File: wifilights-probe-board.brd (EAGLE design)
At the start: 50.8 x 25.4 mm, 18 parts, among them J1 22-05-7028-02, U1 FT232R

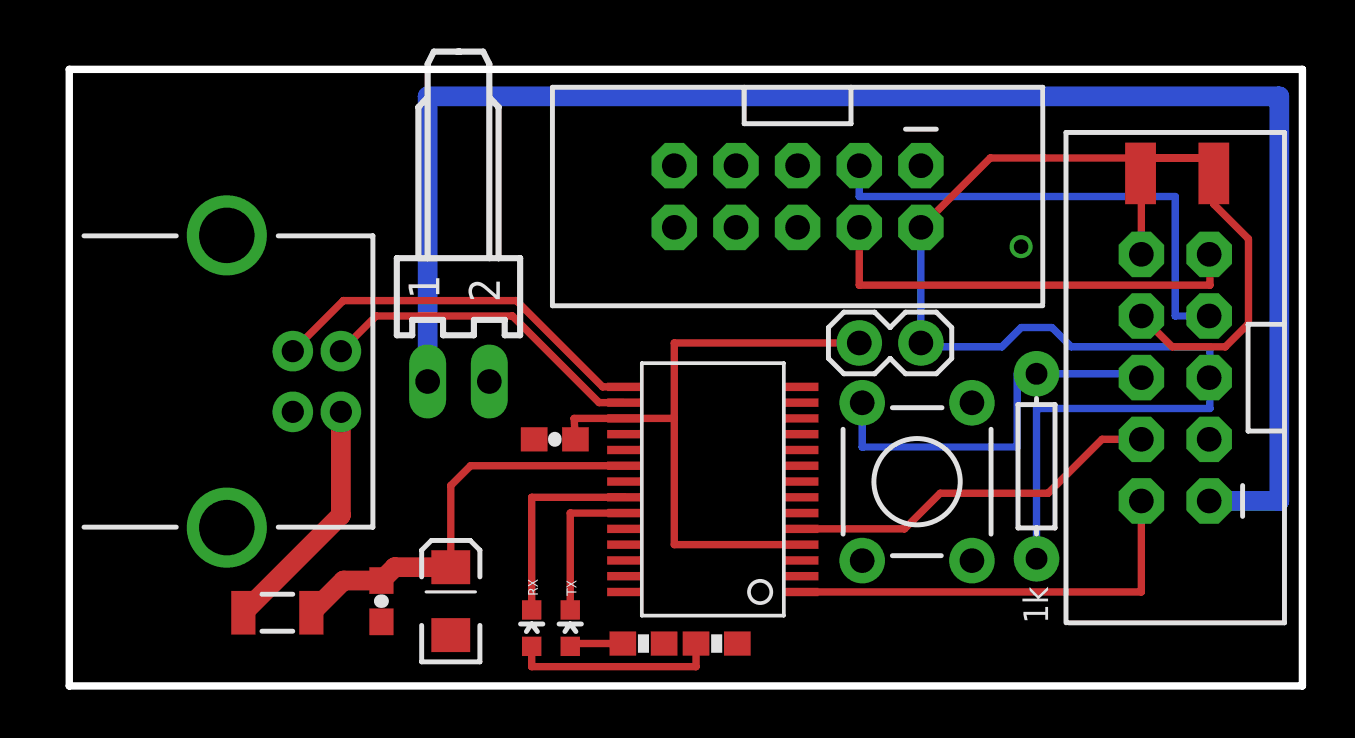
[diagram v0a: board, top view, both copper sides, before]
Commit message: Mk6 complete & DRC'd
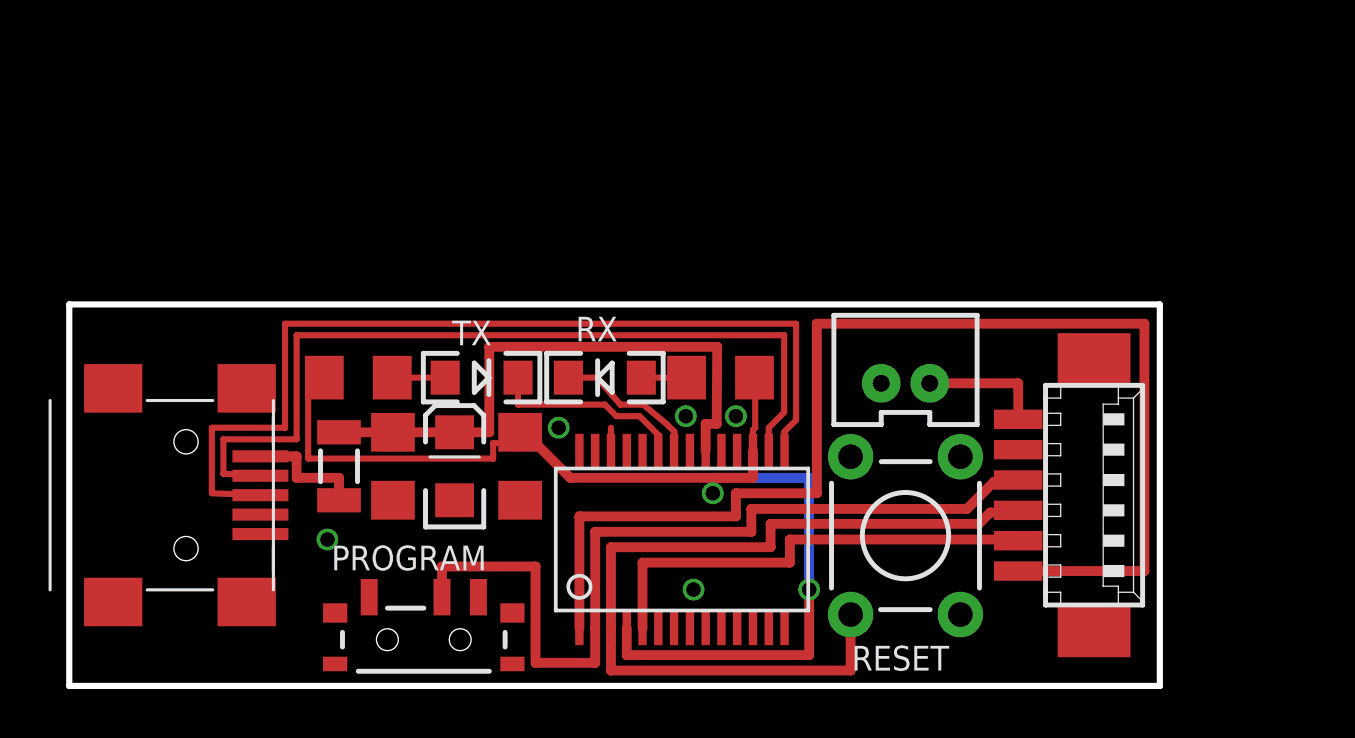
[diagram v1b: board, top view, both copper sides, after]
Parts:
- removed J1: 22-05-7028-02, con-molex:7395-02
- removed JP2: (no value), SparkFun-Connectors:2X5-SHROUDED_LOCK
- removed JP3: (no value), SparkFun-Retired:1X02
- removed JP4: USB-B, SparkFun-Connectors:USB-B-PTH
- removed R4: 1k, SparkFun-Passives:AXIAL-0.3
- removed S2: SWITCH-MOMENTARY-2PTH, SparkFun-Electromechanical:TACTILE-PTH
- removed SH1, SH2: SHORT-HT5, shorts-old:SHORT_TOP-50
- added CN1: (no value), adafruit:USB-MINIB
- added PROGRAM: (no value), SparkFun-Electromechanical:SWITCH-SPST-SMD-A
- added RESET: SWITCH-MOMENTARY-2PTH, SparkFun-Electromechanical:TACTILE-PTH
- added X1: 53261-06, con-molex:53261-06
- C1, C2: device SparkFun-Capacitors:0603-CAP -> SparkFun-Passives:1206
- JP1: value (none) -> 12V DC; device SparkFun-Connectors:2X5-SHROUDED -> SparkFun-Connectors:JST-2-PTH-VERT
- R1, R2: device SparkFun-Resistors:0603-RES -> SparkFun-Passives:1206
- RX: value Green -> GREEN; device SparkFun-LED:LED-0603 -> SparkFun-LED:LED-1206
- TX: value Red -> RED; device SparkFun-LED:LED-0603 -> SparkFun-LED:LED-1206
- moved R1 16.1 mm to (11.9, 12.7), turned to 180 degrees
- moved R2 11.0 mm to (26.8, 12.7)
- moved TX 10.9 mm to (17.0, 12.7)
- moved RX 10.8 mm to (22.1, 12.7), turned to 180 degrees
- moved JP1 8.41 mm to (34.4, 13.0), turned to 0 degrees
- moved F1 6.55 mm to (11.1, 9.05), turned to 90 degrees
- moved C2 5.58 mm to (13.3, 9.05)
- moved C5 5.56 mm to (15.9, 9.05)
- moved U1 2.42 mm to (25.2, 6.03), turned to 0 degrees
- moved C1 1.81 mm to (18.6, 9.05), turned to 270 degrees
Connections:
- removed net 3.3V-INT: C1.1, JP3.2, U1.17, U1.4
- removed net 5V: JP1.1
- removed net CH_PD: JP2.10, SH2.1
- removed net GPIO0: JP2.6, R4.P$1, S2.3
- removed net GPIO2: JP2.8, SH1.1
- removed net N$4: R1.2
- removed net N$5: R2.2
- removed net P_RED: JP1.8
- removed net P_WHITE: JP1.6
- removed net RED: JP1.7
- removed net SCL: JP1.3, JP2.7
- removed net SDA: JP1.4, JP2.9
- removed net WHITE: JP1.5
- net 12V: now also JP1.2, X1.6; no longer J1.1, JP2.1
- net 3.3V: now also C1.1, R1.2, R2.2, U1.17, U1.4; no longer JP1.2, JP2.5, JP3.1, R4.P$2, SH1.2, SH2.2
- net DTR: now also PROGRAM.2, X1.4
- net GND: now also CN1.GND, JP1.1, PROGRAM.3, RESET.3, X1.5; no longer J1.2, JP1.10, JP1.9, JP2.3, JP4.GND, S2.1
- net N$3: now also CN1.VBUS; no longer JP4.VBUS
- net RTS: now also RESET.1, X1.3
- net RXD: now also X1.2; no longer JP2.4
- net TXD: now also X1.1; no longer JP2.2
- net USB_D+: now also CN1.D+; no longer JP4.D+
- net USB_D-: now also CN1.D-; no longer JP4.D-
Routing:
- net 12V: track 66.4 -> 5.13 mm
- net DTR: track 0.00 -> 35.8 mm
- net RTS: track 0.00 -> 35.2 mm
- net TXD: track 17.7 -> 51.2 mm
- net 3.3V-INT: track 26.2 -> 0.00 mm
- net USB_D+: track 16.0 -> 38.5 mm
- net USB_D-: track 13.7 -> 35.4 mm
- net SCL: track 20.6 -> 0.00 mm
- net SDA: track 18.1 -> 0.00 mm
- net GPIO0: track 16.5 -> 0.00 mm
- net GPIO2: track 11.5 -> 0.00 mm
- net N$2: track 8.56 -> 1.86 mm
- net VCC: track 17.4 -> 23.8 mm
- net N$3: track 9.94 -> 5.05 mm
- net RXD: track 15.5 -> 19.2 mm
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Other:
- board size 50.8 x 25.4 mm -> 44.9 x 15.7 mm
